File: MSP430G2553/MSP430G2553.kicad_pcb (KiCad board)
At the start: 2 copper layers, 30 x 30.8 mm, 29 parts, among them J1 Power, J2 Programmer, J3 Conn_01x06_Female, J4 Conn_01x08_Female, SW1 SW_Push, U1 MSP430G2553IPW20, Y1 Crystal_GND24

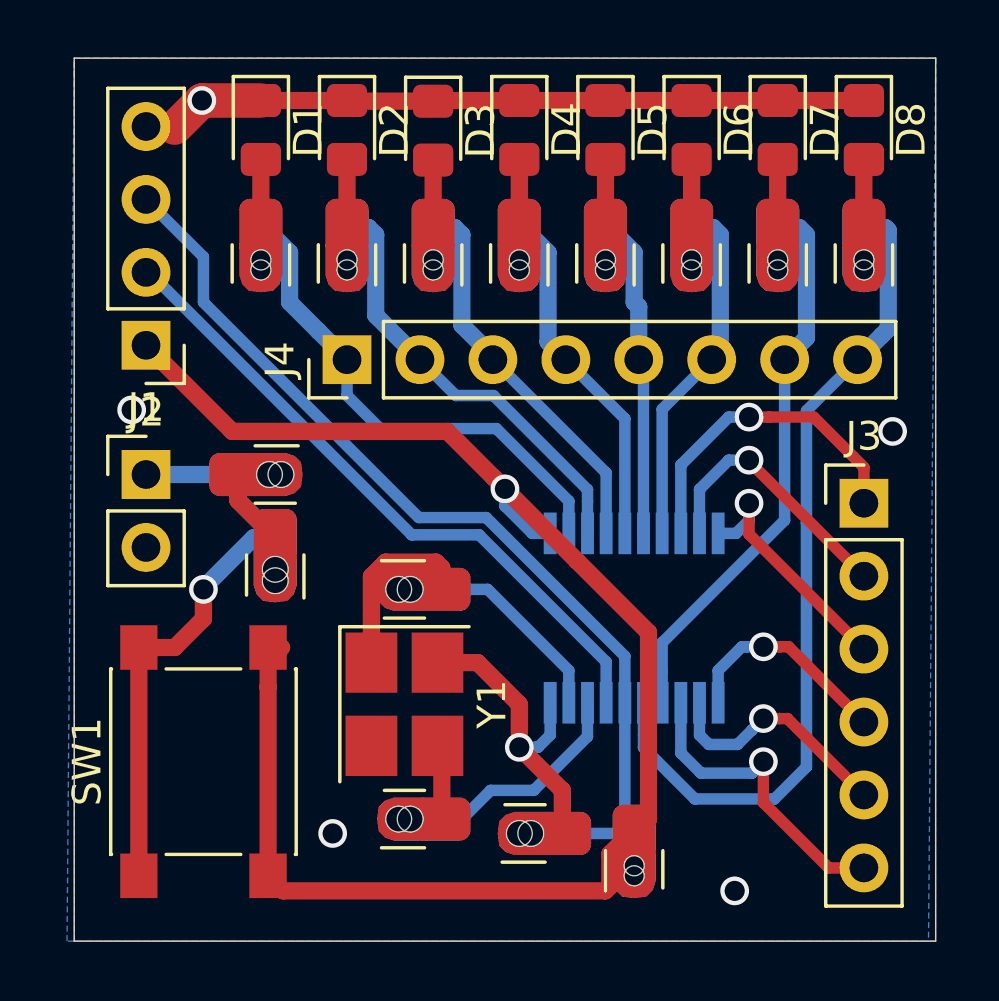
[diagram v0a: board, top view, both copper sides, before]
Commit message: new msp board and array.
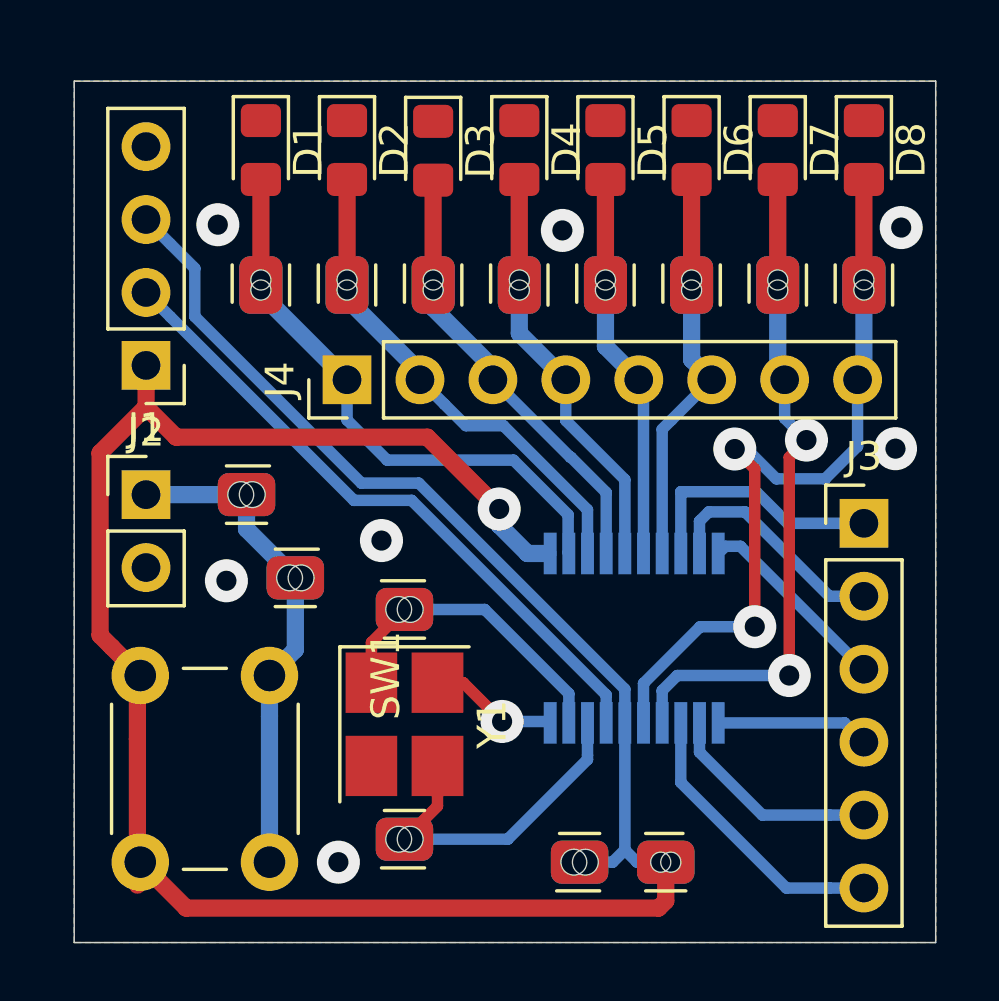
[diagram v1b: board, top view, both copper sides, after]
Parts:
- C1, C2, C3, C4, C5: footprint thSMD:thsmd_03_l -> thSMD:thsmd_04_l
- R1, R2, R3, R4, R5, R6, R7, R8, R9: footprint thSMD:thsmd_03_s -> thSMD:thsmd_04_s
- SW1: footprint Button_Switch_SMD:SW_Push_1P1T_NO_6x6mm_H9.5mm -> Button_Switch_THT:SW_PUSH_6mm
- moved SW1 3.78 mm to (88.3, 91.0), turned to 270 degrees
- moved C4 2.15 mm to (99.1, 97.5)
- moved C3 1.22 mm to (87.5, 84.7)
- moved R1 1.14 mm to (102.1, 97.5), turned to 0 degrees
- moved C2 0.71 mm to (89.2, 87.6), turned to 0 degrees
- moved C1 0.70 mm to (93.0, 88.7)
- moved C5 0.70 mm to (93.0, 96.7)
- moved D1 0.70 mm to (88.0, 72.7)
- moved D2 0.70 mm to (91.0, 72.7)
- moved D4 0.70 mm to (97.0, 72.7)
- moved D5 0.70 mm to (100.0, 72.7)
- moved D6 0.70 mm to (103.0, 72.7)
- moved D7 0.70 mm to (106.0, 72.7)
- moved D8 0.70 mm to (109.0, 72.7)
- moved J1 0.70 mm to (84.0, 84.7)
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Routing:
- net GND: track 38.1 -> 4.50 mm, vias 6 -> 8
- net P1.7: track 29.2 -> 23.4 mm, vias 0 -> 2
- net Net-(C2-Pad1): track 20.9 -> 17.4 mm, vias 1 -> 0
- net Net-(C1-Pad1): track 6.49 -> 3.03 mm
- net P2.0: track 11.4 -> 8.98 mm, vias 1 -> 0
- net P2.3: track 7.63 -> 5.35 mm, vias 1 -> 0
- net P1.5: track 12.3 -> 10.4 mm
- net P1.1: track 15.3 -> 13.6 mm
- net P1.2: track 13.6 -> 11.9 mm
- net P2.2: track 8.60 -> 6.95 mm, vias 1 -> 0
- net P1.4: track 11.3 -> 9.90 mm
- net P1.3: track 12.2 -> 10.9 mm
- net Net-(C5-Pad1): track 7.44 -> 8.80 mm
- net Net-(D8-Pad2): track 2.38 -> 3.68 mm
- net Net-(D7-Pad2): track 2.38 -> 3.68 mm
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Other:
- board size 30 x 30.8 mm -> 30 x 30 mm
